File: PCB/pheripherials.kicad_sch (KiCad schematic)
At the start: 8 parts, among them J4 SM04B-SRSS-TB, Q1 Q_NMOS, U6 SHT4x

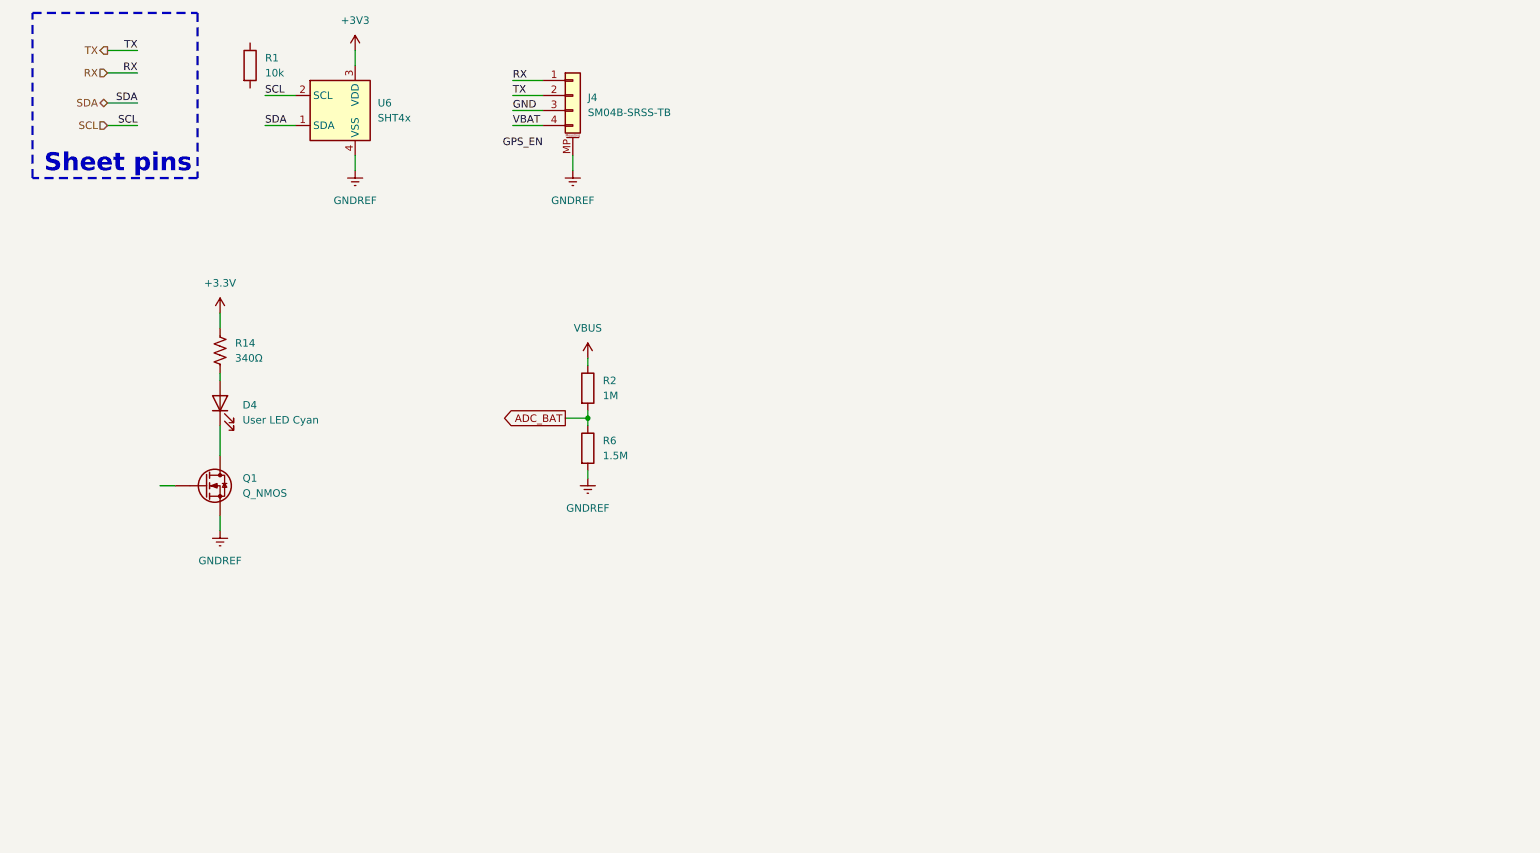
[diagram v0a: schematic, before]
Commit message: a bit of work on the pheripherials
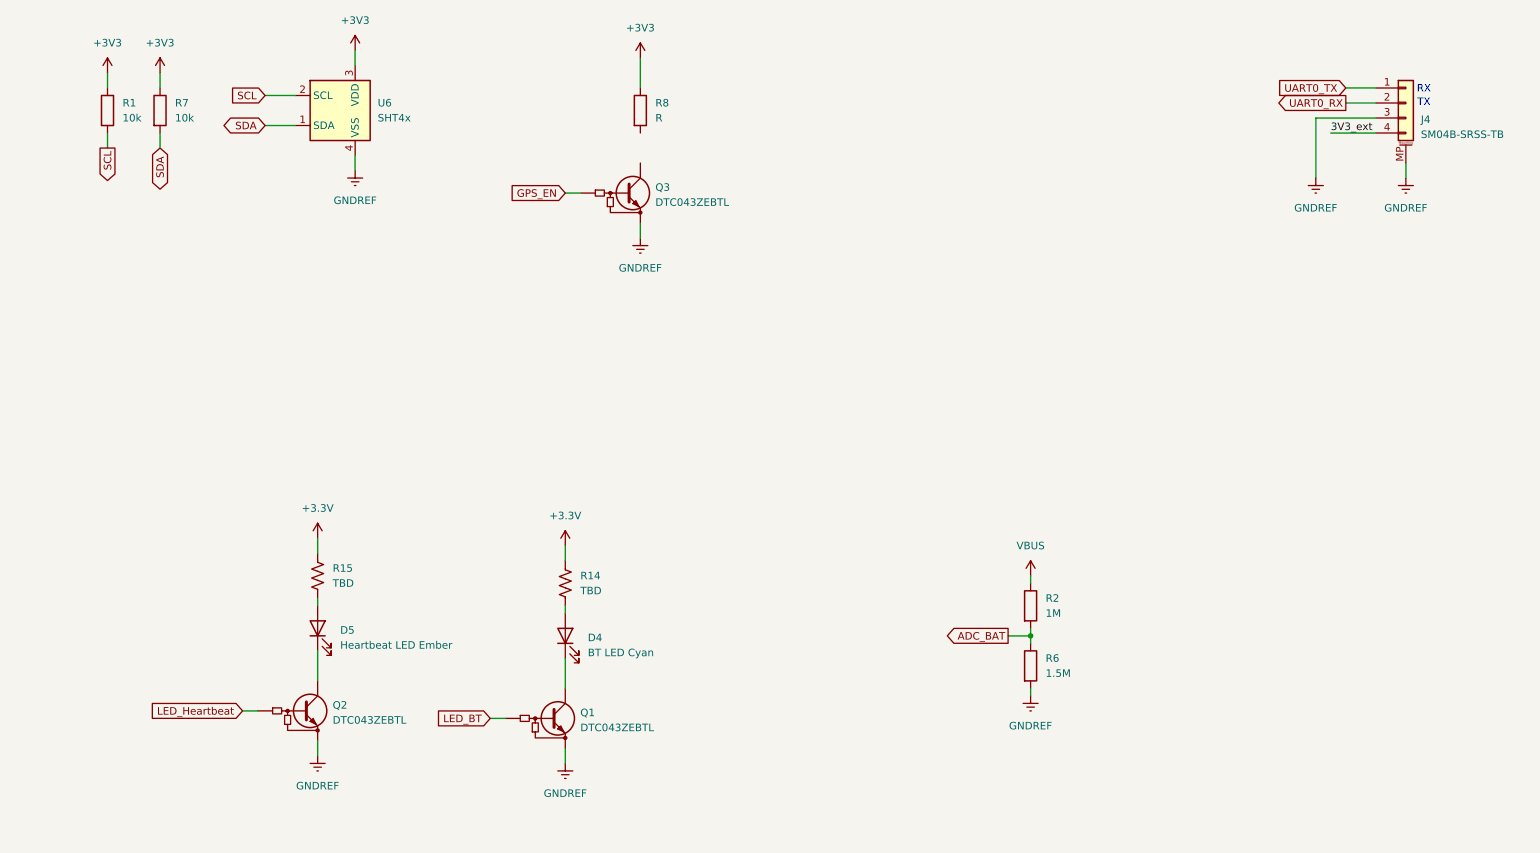
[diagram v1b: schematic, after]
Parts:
- removed Q1: Q_NMOS, Package_DFN_QFN:Nordic_AQFN-94-1EP_7x7mm_P0.4mm, symbol Device:Q_NMOS
- added D5: Heartbeat LED Ember, LED_SMD:LED_0603_1608Metric_Pad1.05x0.95mm_HandSolder, symbol 0_generic_component:LED
- added Q1, Q2, Q3: DTC043ZEBTL, Package_TO_SOT_SMD:SOT-416, symbol Device:Q_NPN_BRT
- added R15: TBD, Resistor_SMD:R_0603_1608Metric_Pad0.98x0.95mm_HandSolder, symbol 0_generic_component:R
- added R7: 10k, symbol Device:R
- added R8: R, symbol Device:R
- D4: value User LED Cyan -> BT LED Cyan
- R14: value 340Ω -> TBD
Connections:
- net GND is gone; now on net GNDREF: J4.3 (Pin_3)
- net +3.3V: now also R15.2
- net +3V3: now also R1.1, R7.1, R8.1
- net GNDREF: now also Q1.E, Q2.E, Q3.E
- net GPS_EN: now also Q3.B
- net SCL: now also R1.2
- net SDA: now also R7.2
- net at D4.1 (K): now also Q1.C
- net RX renamed UART0_TX
- net TX renamed UART0_RX
- net VBAT renamed 3V3_ext
- new net: D5.1 (K), Q2.C
- new net: D5.2 (A), R15.1
- new net LED_BT: Q1.B
- new net LED_Heartbeat: Q2.B
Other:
- note added: "RX"
- note added: "TX"
- moved on the sheet: D4, J4, R1, R14, R2, R6

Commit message: a bit of polishing and work on the pheripherials
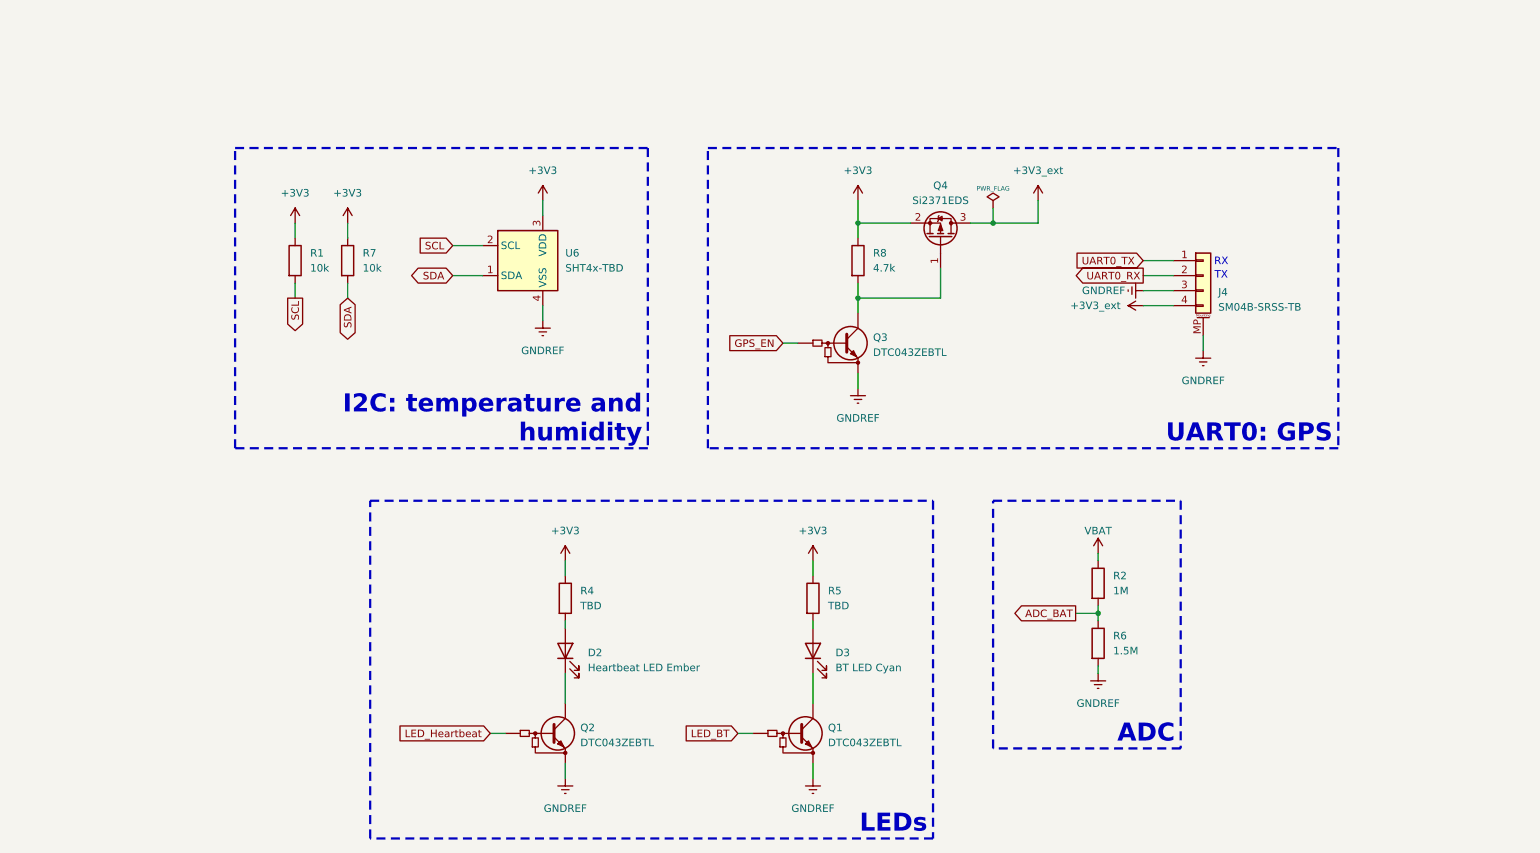
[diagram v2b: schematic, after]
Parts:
- removed D4: BT LED Cyan, LED_SMD:LED_0603_1608Metric_Pad1.05x0.95mm_HandSolder, symbol 0_generic_component:LED
- removed D5: Heartbeat LED Ember, LED_SMD:LED_0603_1608Metric_Pad1.05x0.95mm_HandSolder, symbol 0_generic_component:LED
- removed R14, R15: TBD, Resistor_SMD:R_0603_1608Metric_Pad0.98x0.95mm_HandSolder, symbol 0_generic_component:R
- added D2: Heartbeat LED Ember, symbol Device:LED
- added D3: BT LED Cyan, symbol Device:LED
- added Q4: Si2371EDS, Package_TO_SOT_SMD:SOT-23, symbol Transistor_FET:Si2371EDS
- added R4, R5: TBD, symbol Device:R
- R8: value R -> 4.7k
- U6: value SHT4x -> SHT4x-TBD
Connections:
- net +3V3: now also Q4.2 (S), R4.1, R5.1
- net at Q3.C: now also R8.2, Q4.1 (G)
- net at Q2.C: now also D2.1 (K)
- net at Q1.C: now also D3.1 (K)
- net 3V3_ext renamed +3V3_ext
- net +3V3_ext: now also Q4.3 (D)
- net VBUS renamed VBAT
- new net: D2.2 (A), R4.2
- new net: D3.2 (A), R5.2
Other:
- moved on the sheet: J4, Q1, Q2, Q3, R1, R2, R6, R7, R8, U6
